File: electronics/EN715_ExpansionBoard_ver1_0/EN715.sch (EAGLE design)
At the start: 34 parts, among them IC1 FE1.1S

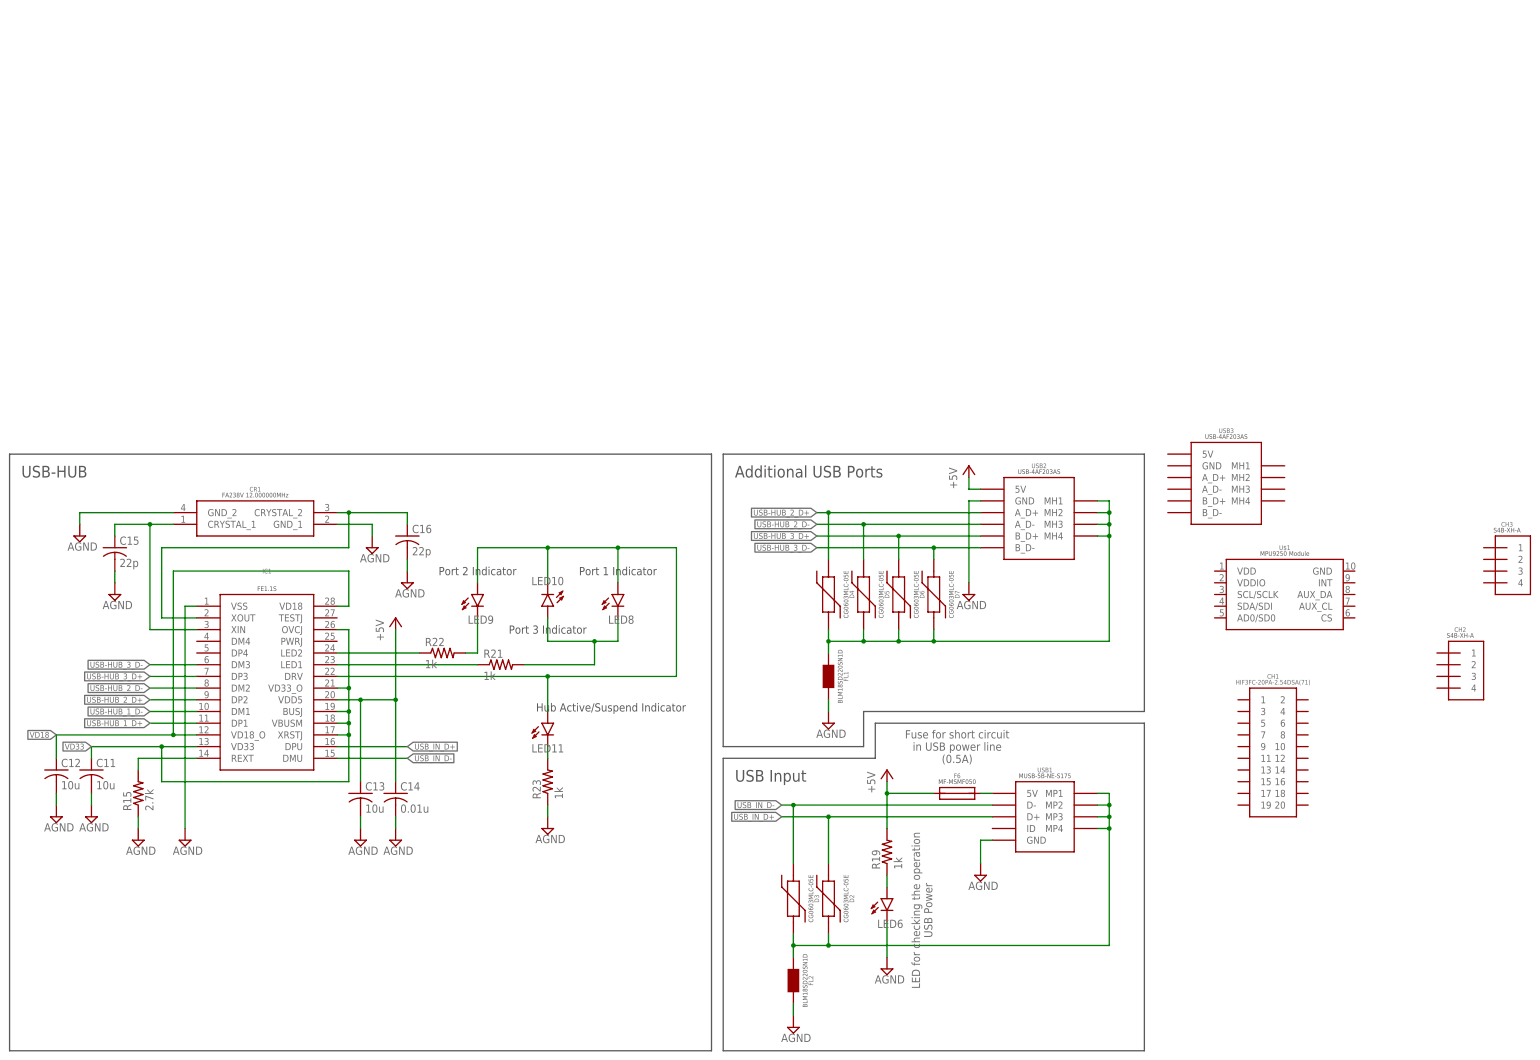
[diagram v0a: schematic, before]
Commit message: Update Expansion board
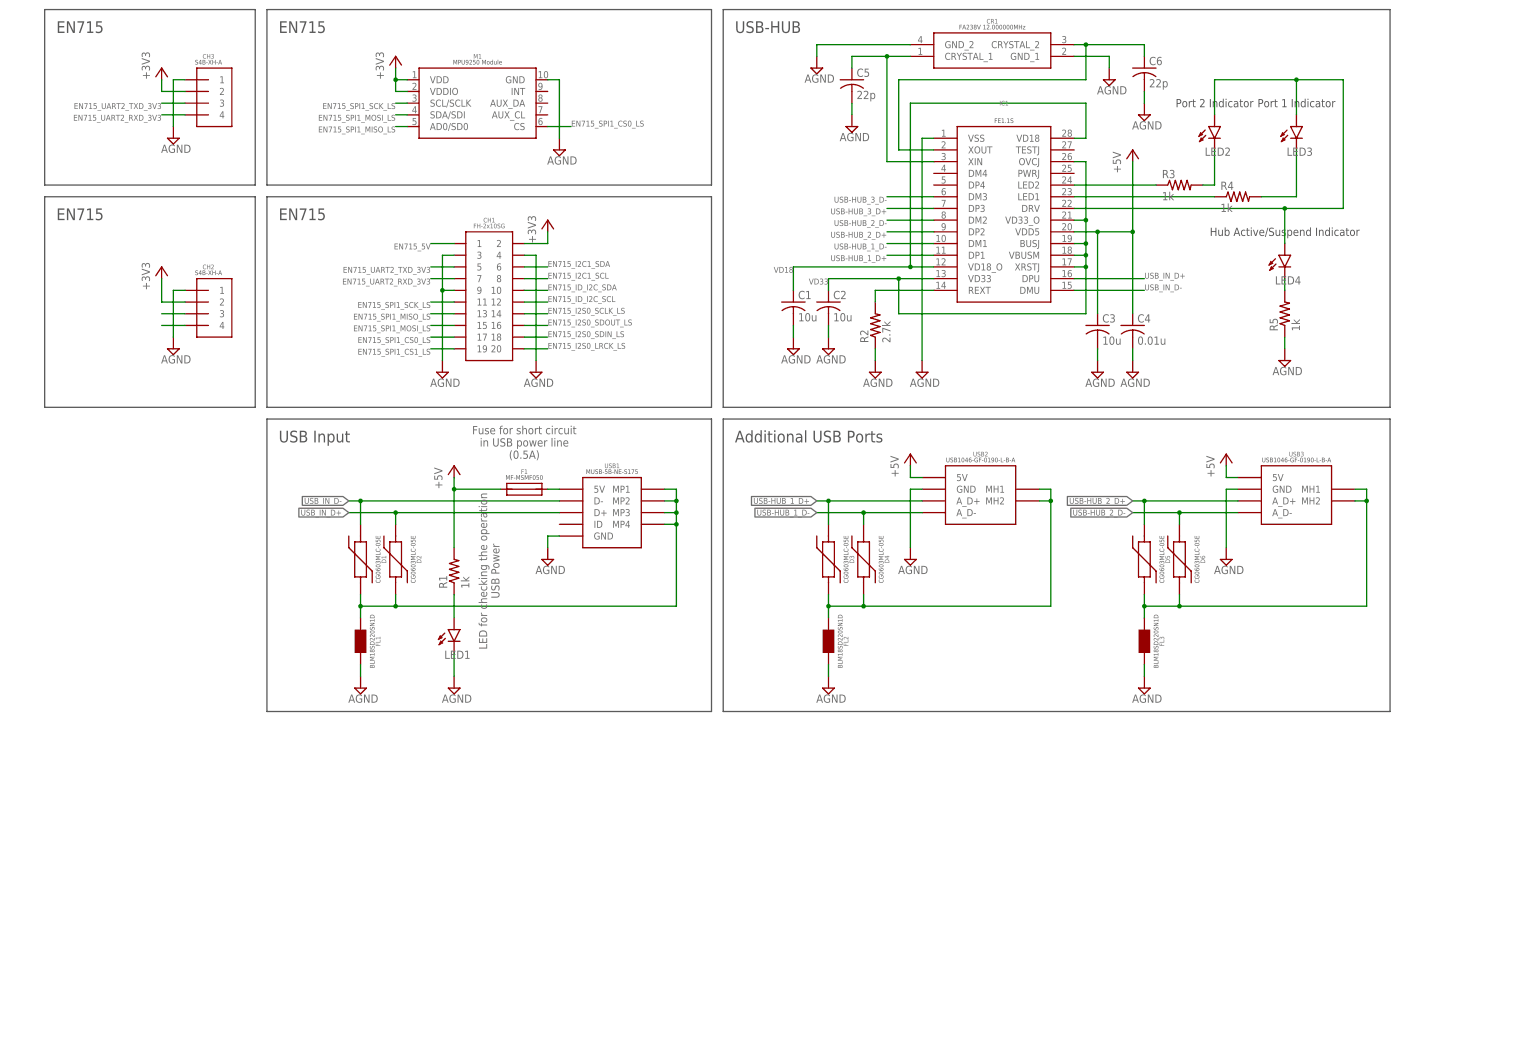
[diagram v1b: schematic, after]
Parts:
- removed C11, C12, C13: 10u, rcl:C-USC0603
- removed C14: 0.01u, rcl:C-USC0603
- removed C15, C16: 22p, rcl:C-USC0603
- removed D7: CG0603MLC-05E, CG0603MLC-05E:CG0603MLC-05E
- removed F6: MF-MSMF050, MF-MSMF:MF-MSMF050
- removed LED10, LED11, LED6, LED8, LED9: (no value), led:LEDSML0603
- removed R15: 2.7k, rcl:R-US_R0603
- removed R19, R21, R22, R23: 1k, rcl:R-US_R0603
- removed U$1: MPU9250_MODULE, Strawberry-Linux_MPUP250_Module:MPU9250_MODULE
- added C1, C2, C3: 10u, rcl:C-USC0603
- added C4: 0.01u, rcl:C-USC0603
- added C5, C6: 22p, rcl:C-USC0603
- added D1: CG0603MLC-05E, CG0603MLC-05E:CG0603MLC-05E
- added F1: MF-MSMF050, MF-MSMF:MF-MSMF050
- added FL3: BLM18SD220SN1D, BLM18SD220SN1D:BLM18SD220SN1D
- added LED1, LED2, LED3, LED4: (no value), led:LEDSML0603
- added M1: MPU9250_MODULE, Strawberry-Linux_MPUP250_Module:MPU9250_MODULE
- added R1, R3, R4, R5: 1k, rcl:R-US_R0603
- added R2: 2.7k, rcl:R-US_R0603
- CH1: value HIF3FC-20PA-2.54DSA(71) -> 2X10; device HiroseConnector:HIF3FC-20PA-2.54DSA(71) -> Pin_socket:2X10
- USB1: value MINI_USB_5P_B_TYPE -> MINI_USB_B_SMD; device USB_Connector:MINI_USB_5P_B_TYPE -> USB_Connector:MINI_USB_B_SMD
- USB2, USB3: value USB_4P_A_TYPE_X2 -> USB_A_X1_SMD; device USB_Connector:USB_4P_A_TYPE_X2 -> USB_Connector:USB_A_X1_SMD
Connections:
- removed net USB_A_SHIELD: D4.2, D5.2, D6.2, D7.2, FL1.1, USB2.MH1, USB2.MH2, USB2.MH3, USB2.MH4
- new net +3V3: CH1.2, CH2.2, CH3.2, M1.VDD, M1.VDDIO
- new net EN715_5V: CH1.1
- new net EN715_I2C1_SCL: CH1.8
- new net EN715_I2C1_SDA: CH1.6
- new net EN715_I2S0_LRCK_LS: CH1.20
- new net EN715_I2S0_SCLK_LS: CH1.14
- new net EN715_I2S0_SDIN_LS: CH1.18
- new net EN715_I2S0_SDOUT_LS: CH1.16
- new net EN715_ID_I2C_SCL: CH1.12
- new net EN715_ID_I2C_SDA: CH1.10
- new net EN715_SPI1_CS0_LS: CH1.17, M1.CS
- new net EN715_SPI1_CS1_LS: CH1.19
- new net EN715_SPI1_MISO_LS: CH1.13, M1.AD0/SD0
- new net EN715_SPI1_MOSI_LS: CH1.15, M1.SDA/SDI
- new net EN715_SPI1_SCK_LS: CH1.11, M1.SCL/SCLK
- new net EN715_UART2_RXD_3V3: CH1.7, CH3.4
- new net EN715_UART2_TXD_3V3: CH1.5, CH3.3
- new net N$1: CH2.3
- new net N$2: CH2.4
- new net USB_A_1_SHIELD: D3.2, D4.2, FL2.1, USB2.MH1, USB2.MH2
- new net USB_A_2_SHIELD: D5.2, D6.2, FL3.1, USB3.MH1, USB3.MH2
- net +5V: now also C3.1, C4.1, F1.1, R1.2, USB3.5V; no longer C13.1, C14.1, F6.1, R19.2
- net AGND: now also C1.2, C2.2, C3.2, C4.2, C5.2, C6.2, CH1.3, CH1.4, CH1.9, CH2.1, CH3.1, FL3.2, LED1.C, M1.GND, R2.1, R5.1, USB3.GND; no longer C11.2, C12.2, C13.2, C14.2, C15.2, C16.2, LED6.C, R15.1, R23.1
- net B_FUSE_USB_MINI_B: now also F1.2; no longer F6.2
- net FE1.1S_DRV: now also LED2.A, LED3.A, LED4.A; no longer LED10.C, LED11.A, LED8.A, LED9.A
- net FE1.1S_DRV_LED_A: now also LED4.C, R5.2; no longer LED11.C, R23.2
- net FE1.1S_LED1_A: now also LED3.C, R4.2; no longer LED10.A, LED8.C, R21.2
- net FE1.1S_LED_1_B: now also R4.1; no longer R21.1
- net FE1.1S_LED_2_A: now also LED2.C, R3.2; no longer LED9.C, R22.2
- net FE1.1S_LED_2_B: now also R3.1; no longer R22.1
- net LED_USBIN: now also LED1.A, R1.1; no longer LED6.A, R19.1
- net REXT_FE1.1S: now also R2.2; no longer R15.2
- net USB-HUB_1_D+: now also D3.1, USB2.A_D+
- net USB-HUB_1_D-: now also D4.1, USB2.A_D-
- net USB-HUB_2_D+: now also D5.1, USB3.A_D+; no longer D4.1, USB2.A_D+
- net USB-HUB_2_D-: now also D6.1, USB3.A_D-; no longer D5.1, USB2.A_D-
- net USB-HUB_3_D+: no longer D6.1, USB2.B_D+
- net USB-HUB_3_D-: no longer D7.1, USB2.B_D-
- net USB_IN_D-: now also D1.1; no longer D3.1
- net USB_MINI_B_SHIELD: now also D1.2, FL1.1; no longer D3.2, FL2.1
- net VD18: now also C1.1; no longer C12.1
- net VD33: now also C2.1; no longer C11.1
- net XIN_FE1.1S: now also C5.1; no longer C15.1
- net XOUT_FE1.1S: now also C6.1; no longer C16.1
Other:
- note added: "EN715"
- note removed: "Port 3 Indicator"
- moved on the sheet: CH1, CH2, CH3, CR1, D2, D3, D4, D5, D6, FL1, FL2, IC1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
